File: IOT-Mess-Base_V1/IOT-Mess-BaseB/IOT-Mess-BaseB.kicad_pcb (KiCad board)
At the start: 2 copper layers, 92.7 x 40 mm, 9 parts, among them J1 Milk-V Duo, J3 Conn_01x19_Pin, J4 Lolin32-Lite, J6 Conn_01x36_Pin, J8 Luat32 C3, SW3 SW_Push

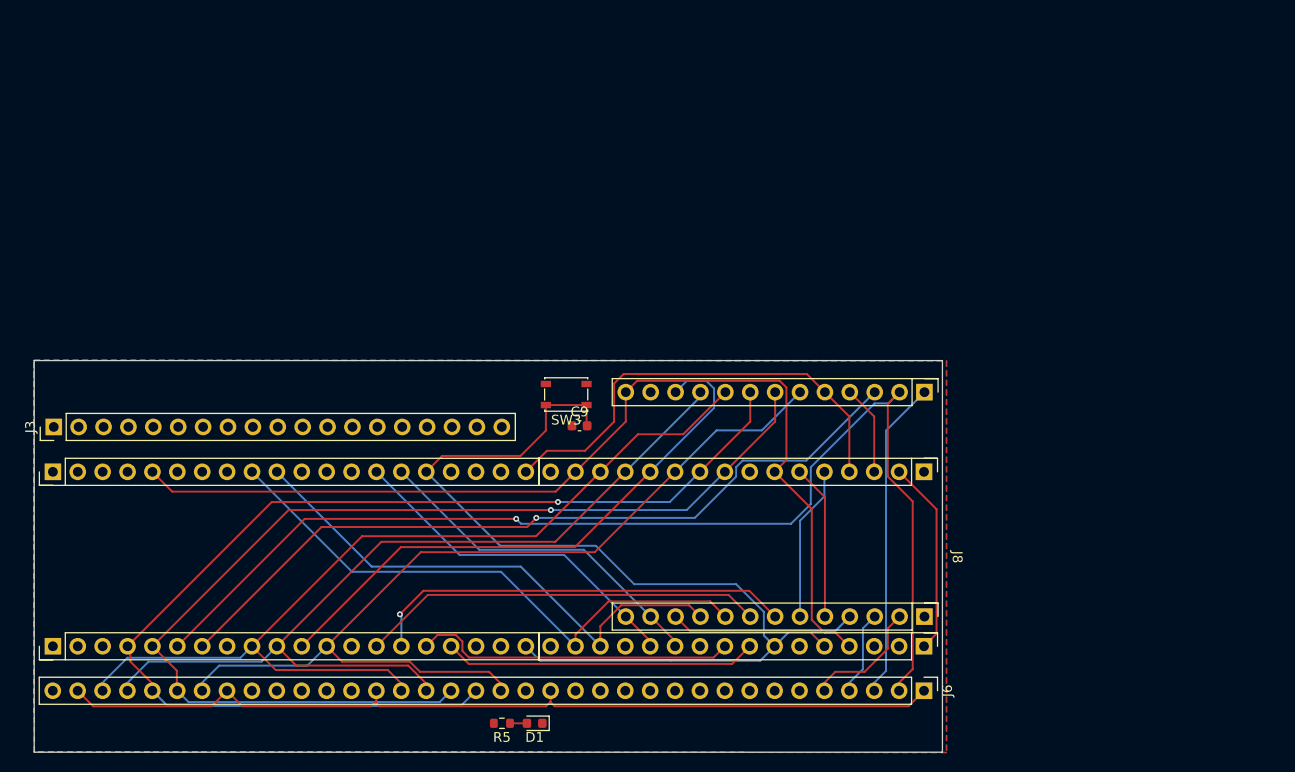
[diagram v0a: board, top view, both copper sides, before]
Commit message: did some works.
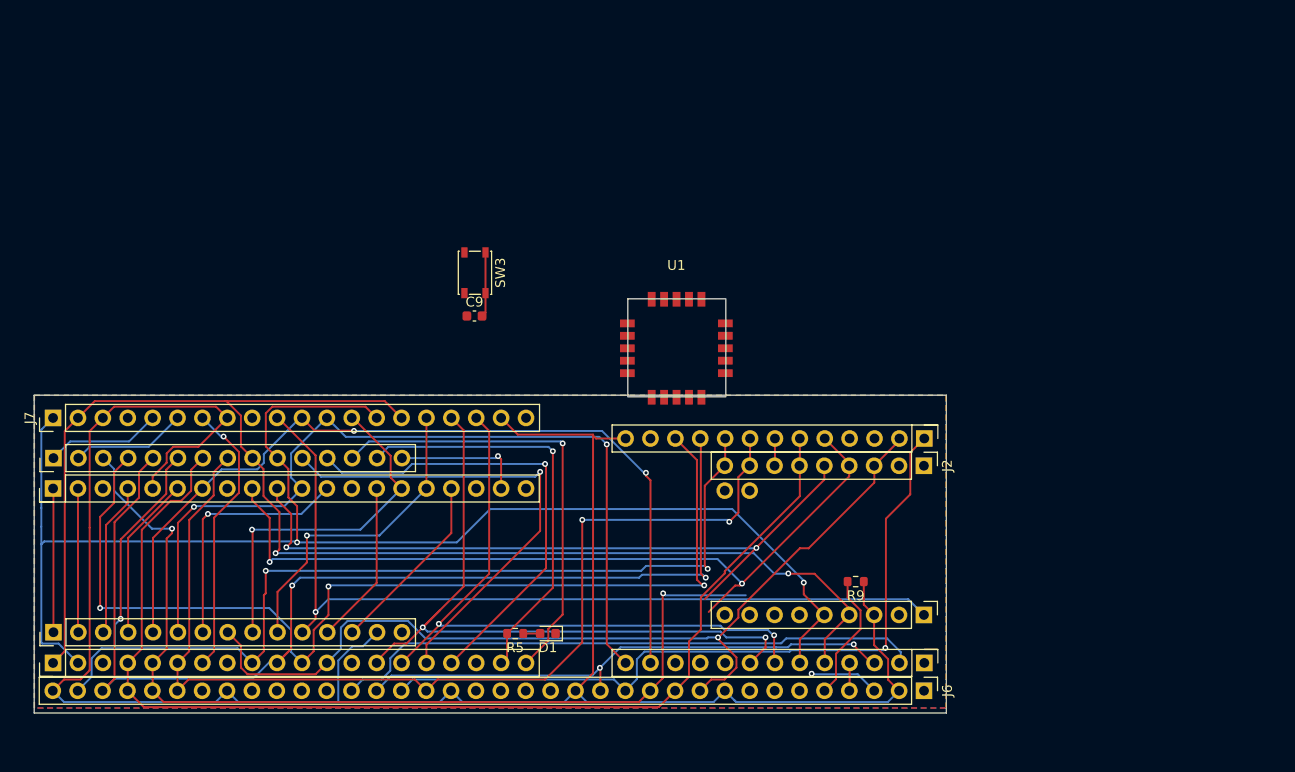
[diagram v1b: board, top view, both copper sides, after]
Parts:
- removed J8: Luat32 C3, IOT-Mess-Footprints:Luat32 C3
- added J2: SuperMini_ESP32-H2, IOT-Mess-Footprints:SuperMiniH2, F.Cu at (161.1, 112.6)
- added J7: Conn_01x20_Pin, Connector_PinHeader_2.54mm:PinHeader_1x20_P2.54mm_Vertical, F.Cu at (72.2, 107.7)
- added R9: 10K, Resistor_SMD:R_0603_1608Metric, F.Cu at (154.1, 124.4)
- added U1: ~, IOT-Mess-Footprints:E220-900, F.Cu at (135.8, 100.1)
- J3: value Conn_01x19_Pin -> CH_P20; footprint Connector_PinHeader_2.54mm:PinHeader_1x19_P2.54mm_Vertical -> IOT-Mess-Footprints:CH_P20
- moved J3 21.0 mm to (72.2, 129.6)
- moved SW3 15.5 mm to (115.2, 92.9), turned to -90 degrees
- moved C9 15.5 mm to (115.2, 97.3)
- moved D1 9.25 mm to (122.7, 129.7)
- moved R5 9.25 mm to (119.4, 129.7)
- moved J4 4.73 mm to (161.1, 109.8)
- moved J1 1.70 mm to (72.2, 132.7)
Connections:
- C9 pad 2: ROT_SW -> M20
- J1 pad 12: CS_0 -> CS_1
- J1 pad 16: TX0 -> M16
- J1 pad 17: RX0 -> M17
- J1 pad 19: Net-(J1-Pin_19) -> M19
- J1 pad 20: ROT_SW -> M20
- J1 pad 21: WLED -> M21
- J1 pad 22: unconnected-(J1-Pin_22-Pad22) -> M22
- J1 pad 24: unconnected-(J1-Pin_24-Pad24) -> M24
- J1 pad 25: ROT_SW -> DONE
- J1 pad 26: ROT_B -> DRIVE
- J1 pad 27: ROT_A -> M27
- J1 pad 29: unconnected-(J1-Pin_29-Pad29) -> M29
- J1 pad 34: unconnected-(J1-Pin_34-Pad34) -> LSW0
- J1 pad 35: unconnected-(J1-Pin_35-Pad35) -> M35
- J1 pad 4: RST1 -> DC
- J1 pad 5: DC -> RST1
- J1 pad 6: CS_1 -> CS_0
- J1 pad 7: CS_2 -> L7
- J4 pad 0: BOOT -> unconnected-(J4-Pin_4a-Pad0)
- J4 pad 16: CS_0 -> DC
- J4 pad 17: DC -> RST1
- J4 pad 22: LED22 -> unconnected-(J4-Pin_12a-Pad22)
- J4 pad 27: ROT_SW -> ADC_Y
- J4 pad 34*: ADC_Y -> unconnected-(J4-Pin_10b-Pad34*)
- J4 pad 35*: ADC_X -> unconnected-(J4-Pin_9b-Pad35*)
- J4 pad 36*: ROT_B -> LSW0
- J4 pad 39*: ROT_A -> LSW1
- J4 pad 3V: VCC -> +3.3V
- J4 pad 4: WLED -> ADC_X
- J4 pad 5: RST1 -> CS_0
- J4 pad EN: RST0 -> unconnected-(J4-Pin_11b-PadEN)
- J6 pad 1: +3.3V -> GND
- J6 pad 10: unconnected-(J6-Pin_10-Pad10) -> CS_1
- J6 pad 11: unconnected-(J6-Pin_11-Pad11) -> DC
- J6 pad 12: unconnected-(J6-Pin_12-Pad12) -> RST1
- J6 pad 13: unconnected-(J6-Pin_13-Pad13) -> MOSI_1
- J6 pad 14: unconnected-(J6-Pin_14-Pad14) -> SCK_1
- J6 pad 15: unconnected-(J6-Pin_15-Pad15) -> +3.3V
- J6 pad 16: +3.3V -> GND
- J6 pad 17: GND -> unconnected-(J6-Pin_17-Pad17)
- J6 pad 18: CS_0 -> unconnected-(J6-Pin_18-Pad18)
- J6 pad 19: RST1 -> unconnected-(J6-Pin_19-Pad19)
- J6 pad 2: CS_1 -> +3.3V
- J6 pad 20: DC -> +3.3V
- J6 pad 21: MOSI_0 -> CS_0
- J6 pad 22: SCK_0 -> MOSI_1
- J6 pad 23: +3.3V -> SCK_1
- J6 pad 24: unconnected-(J6-Pin_24-Pad24) -> MISO_1
- J6 pad 25: unconnected-(J6-Pin_25-Pad25) -> GND
- J6 pad 3: MOSI_1 -> ADC_X
- J6 pad 30: CS_0 -> GND
- J6 pad 31: DC -> CS_0
- J6 pad 33: MOSI_0 -> DC
- J6 pad 34: SCK_0 -> MOSI_0
- J6 pad 35: +3.3V -> SCK_0
- J6 pad 36: GND -> +3.3V
- J6 pad 4: SCK_1 -> ADC_Y
- J6 pad 5: MISO_1 -> ADC_SW
- J6 pad 6: GND -> unconnected-(J6-Pin_6-Pad6)
- J6 pad 9: unconnected-(J6-Pin_9-Pad9) -> +3.3V
- R5 pad 2: Net-(J1-Pin_19) -> M19
- SW3 pad 1: ROT_SW -> M20
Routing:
- net SDA_0: track 15.8 -> 147.3 mm, vias 0 -> 2
- net SCL_0: track 15.9 -> 146.5 mm, vias 0 -> 2
- net +3.3V: track 92.1 -> 210.5 mm
- net VCC: track 103.0 -> 0.00 mm
- net ROT_SW: track 102.8 -> 0.00 mm
- net 5V: track 0.00 -> 87.6 mm, vias 0 -> 1
- net LSW0: track 0.00 -> 87.4 mm, vias 0 -> 2
- net LSW1: track 0.00 -> 87.2 mm, vias 0 -> 2
- net CS_2: track 79.9 -> 0.00 mm, vias 1 -> 0
- net M20: track 0.00 -> 52.8 mm, vias 0 -> 1
- net M16: track 0.00 -> 49.6 mm, vias 0 -> 1
- net MISO_1: track 11.7 -> 60.7 mm
- net SCK_1: track 7.88 -> 56.0 mm, vias 0 -> 2
- net M17: track 0.00 -> 47.6 mm, vias 0 -> 1
- net WLED: track 46.9 -> 0.00 mm
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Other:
- board size 92.7 x 40 mm -> 93.1 x 32.4 mm

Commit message: did some works.
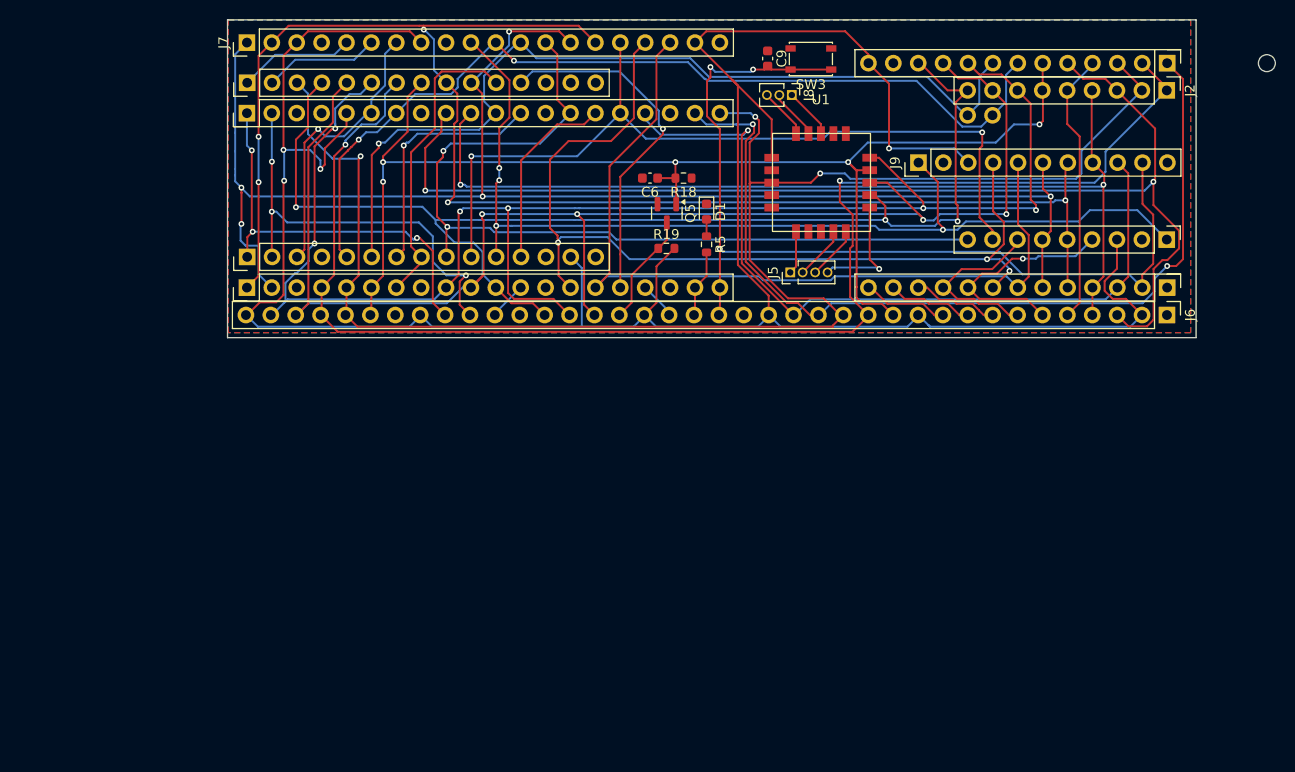
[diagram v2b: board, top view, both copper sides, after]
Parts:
- removed R9: 10K, Resistor_SMD:R_0603_1608Metric
- added C6: C, Capacitor_SMD:C_0603_1608Metric, F.Cu at (133.1, 83.2)
- added J5: Conn_01x04_Pin, Connector_PinHeader_1.27mm:PinHeader_1x04_P1.27mm_Vertical, F.Cu at (147.4, 92.8)
- added J8: Conn_01x03_Pin, Connector_PinHeader_1.27mm:PinHeader_1x03_P1.27mm_Vertical, F.Cu at (147.6, 74.8)
- added J9: Conn_01x11_Pin, Connector_PinHeader_2.54mm:PinHeader_1x11_P2.54mm_Vertical, F.Cu at (160.5, 81.7)
- added Q5: AO3400A, Package_TO_SOT_SMD:SOT-23, F.Cu at (134.8, 86.8)
- added R18: R, Resistor_SMD:R_0603_1608Metric, F.Cu at (136.5, 83.2)
- added R19: R, Resistor_SMD:R_0603_1608Metric, F.Cu at (134.8, 90.4)
- J6: value Conn_01x36_Pin -> Conn_01x38_Pin; footprint Connector_PinHeader_2.54mm:PinHeader_1x36_P2.54mm_Vertical -> Connector_PinHeader_2.54mm:PinHeader_1x38_P2.54mm_Vertical
- moved D1 46.0 mm to (138.9, 86.7), turned to -90 degrees
- moved J6 45.7 mm to (185.9, 97.2)
- moved J2 45.6 mm to (185.8, 74.3)
- moved J4 45.6 mm to (185.9, 71.5)
- moved R5 44.3 mm to (138.9, 90.0), turned to -90 degrees
- moved J7 43.1 mm to (92.0, 69.4)
- moved J1 43.1 mm to (92.0, 94.4)
- moved J3 43.1 mm to (92.0, 91.3)
- moved SW3 40.6 mm to (149.5, 71.1), turned to 180 degrees
- moved C9 39.8 mm to (145.1, 71.0), turned to -90 degrees
- moved U1 22.4 mm to (150.5, 83.2)
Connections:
- net L5 renamed K5
- net L6 renamed K6
- J1 pad 12: CS_1 -> M12
- J1 pad 21: M21 -> RST1
- J1 pad 22: M22 -> MOSI_1
- J1 pad 24: M24 -> SCK_1
- J1 pad 26: DRIVE -> M27
- J1 pad 27: M27 -> DRIVE
- J1 pad 7: L7 -> M7
- J1 pad EN: M37 -> unconnected-(J1-Pin_37-PadEN)
- J2 pad 0: CS_1 -> ADC_X
- J2 pad 1: ADC_X -> ADC_Y
- J2 pad 10: unconnected-(J2-Pin_11-Pad10) -> DONE
- J2 pad 11: unconnected-(J2-Pin_12-Pad11) -> J7
- J2 pad 12: unconnected-(J2-Pin_13-Pad12) -> SDA_0
- J2 pad 13: SDA_0 -> SCL_0
- J2 pad 14: SCL_0 -> J6
- J2 pad 2: ADC_Y -> ADC_SW
- J2 pad 23: unconnected-(J2-Pin_2-Pad23) -> RST1
- J2 pad 24: unconnected-(J2-Pin_1-Pad24) -> DC
- J2 pad 26: unconnected-(J2-Pin_2-Pad26) -> LSW0
- J2 pad 27: unconnected-(J2-Pin_1-Pad27) -> LSW1
- J2 pad 3: DC -> CS_0
- J2 pad 4: RST1 -> SCK_0
- J2 pad 5: CS_0 -> MOSI_0
- J2 pad 8: SCK_0 -> MISO_0
- J2 pad 9: unconnected-(J2-Pin_10-Pad9) -> DRIVE
- J3 pad CC2: M24 -> unconnected-(J3-Pin_13-PadCC2)
- J3 pad D+: M22 -> unconnected-(J3-Pin_30-PadD+)
- J3 pad D-: M19 -> unconnected-(J3-Pin_29-PadD-)
- J3 pad P3: M37 -> M35
- J3 pad P4: M35 -> unconnected-(J3-Pin_4-PadP4)
- J3 pad P8: CS_1 -> M7
- J3 pad RST: M16 -> M7
- J3 pad XI: M17 -> M16
- J3 pad XO: M20 -> unconnected-(J3-Pin_28-PadXO)
- J4 pad 0: unconnected-(J4-Pin_4a-Pad0) -> ADC_SW
- J4 pad 12: MISO_1 -> M20
- J4 pad 15: CS_1 -> DC
- J4 pad 16: DC -> CS_0
- J4 pad 17: RST1 -> LSW0
- J4 pad 2: CS_2 -> RST1
- J4 pad 34*: unconnected-(J4-Pin_10b-Pad34*) -> J7
- J4 pad 35*: unconnected-(J4-Pin_9b-Pad35*) -> J6
- J4 pad 36*: LSW0 -> J9
- J4 pad 39*: LSW1 -> J10
- J4 pad 5: CS_0 -> LSW1
- J4 pad EN: unconnected-(J4-Pin_11b-PadEN) -> J8
- J6 pad 10: CS_1 -> J10
- J6 pad 11: DC -> +3.3V
- J6 pad 12: RST1 -> CS_0
- J6 pad 13: MOSI_1 -> DC
- J6 pad 14: SCK_1 -> RST1
- J6 pad 15: +3.3V -> MOSI_1
- J6 pad 16: GND -> SCK_1
- J6 pad 17: unconnected-(J6-Pin_17-Pad17) -> +3.3V
- J6 pad 18: unconnected-(J6-Pin_18-Pad18) -> GND
- J6 pad 19: unconnected-(J6-Pin_19-Pad19) -> M20
- J6 pad 20: +3.3V -> M19
- J6 pad 21: CS_0 -> M17
- J6 pad 22: MOSI_1 -> +3.3V
- J6 pad 23: SCK_1 -> CS_X
- J6 pad 24: MISO_1 -> MOSI_0
- J6 pad 25: GND -> SCK_0
- J6 pad 26: unconnected-(J6-Pin_26-Pad26) -> MISO_0
- J6 pad 27: unconnected-(J6-Pin_27-Pad27) -> GND
- J6 pad 28: unconnected-(J6-Pin_28-Pad28) -> M12
- J6 pad 29: +3.3V -> M39
- J6 pad 30: GND -> M40
- J6 pad 31: CS_0 -> +3.3V
- J6 pad 32: RST1 -> GND
- J6 pad 33: DC -> CS_0
- J6 pad 34: MOSI_0 -> RST1
- J6 pad 35: SCK_0 -> DC
- J6 pad 36: +3.3V -> MOSI_0
- J6 pad 6: unconnected-(J6-Pin_6-Pad6) -> J6
- J6 pad 7: unconnected-(J6-Pin_7-Pad7) -> J7
- J6 pad 8: unconnected-(J6-Pin_8-Pad8) -> J8
- J6 pad 9: +3.3V -> J9
- J7 pad 7: L7 -> M35
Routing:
- net CS_1: track 94.6 -> 0.00 mm, vias 1 -> 0
- net MISO_1: track 60.7 -> 0.00 mm
- net RST1: track 102.4 -> 161.7 mm, vias 2 -> 3
- net DONE: track 32.5 -> 84.4 mm, vias 1 -> 2
- net DRIVE: track 36.9 -> 87.6 mm, vias 1 -> 2
- net +3.3V: track 210.5 -> 258.7 mm, vias 0 -> 4
- net M20: track 52.8 -> 97.3 mm, vias 1 -> 3
- net M17: track 47.6 -> 3.81 mm, vias 1 -> 0
- net SCK_0: track 113.1 -> 156.5 mm, vias 3 -> 6
- net M19: track 42.4 -> 6.92 mm, vias 1 -> 0
- net MOSI_0: track 112.5 -> 146.5 mm, vias 2 -> 4
- net ADC_X: track 89.7 -> 121.7 mm, vias 3 -> 2
- net M7: track 0.00 -> 30.9 mm
- net M39: track 14.7 -> 43.5 mm, vias 0 -> 3
- net L7: track 28.2 -> 0.00 mm, vias 1 -> 0
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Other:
- board size 93.1 x 32.4 mm -> 98.8 x 32.4 mm
